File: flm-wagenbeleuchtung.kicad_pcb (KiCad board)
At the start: 2 copper layers, 153 x 9.4 mm, 31 parts

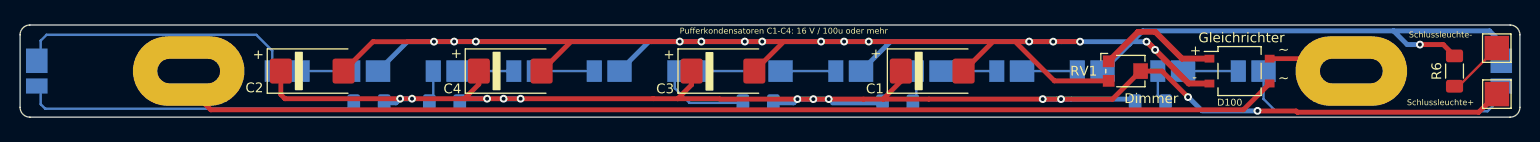
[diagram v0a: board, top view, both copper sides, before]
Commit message: v2
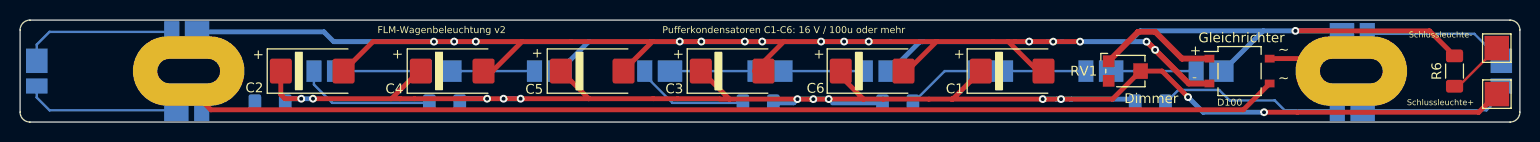
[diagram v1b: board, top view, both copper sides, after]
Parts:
- added C5: 200u, Capacitor_Tantalum_SMD:CP_EIA-7343-31_Kemet-D_Pad2.25x2.55mm_HandSolder, F.Cu at (128.4, 124.7)
- added C6: 200u, Capacitor_Tantalum_SMD:CP_EIA-7343-31_Kemet-D_Pad2.25x2.55mm_HandSolder, F.Cu at (156.9, 124.7)
- moved D32 25.5 mm to (71.7, 124.7), turned to -90 degrees
- moved D42 25.3 mm to (221.1, 124.7), turned to -90 degrees
- moved D31 18.9 mm to (87.0, 120.7)
- moved D43 18.7 mm to (205.9, 128.7)
- moved D33 15.8 mm to (87.0, 128.7), turned to 0 degrees
- moved D41 15.7 mm to (205.9, 120.9), turned to 0 degrees
- moved D23 12.2 mm to (101.5, 124.7)
- moved D1 12.1 mm to (191.5, 124.7)
- moved R4 10.1 mm to (95.5, 127.9)
- moved D22 9.14 mm to (112.8, 124.7)
- moved D2 9.09 mm to (180.2, 124.7)
- moved C1 8.15 mm to (171.2, 124.7)
- moved D21 6.10 mm to (124.0, 124.7)
- moved D3 6.05 mm to (169.0, 124.7)
- moved C4 5.92 mm to (114.1, 124.7)
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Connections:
- RV1 pad 3: GND -> unconnected-(RV1-Pad3)
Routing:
- net Net-(D33-Pad2): track 34.2 -> 5.74 mm
- net Net-(D43-Pad2): track 3.57 -> 18.9 mm
- net Net-(D41-Pad2): track 29.2 -> 14.8 mm
- net Net-(D32-Pad2): track 28.7 -> 16.0 mm
- net Net-(D23-Pad2): track 3.41 -> 13.9 mm
- net Net-(D31-Pad2): track 5.64 -> 16.0 mm
- net Net-(D42-Pad2): track 5.64 -> 15.7 mm
- net GND: track 250.5 -> 260.3 mm
- net VCC: track 169.5 -> 178.2 mm
- net Net-(D3-Pad2): track 3.39 -> 7.74 mm
- net Net-(D21-Pad2): track 5.64 -> 8.67 mm
- net Net-(D22-Pad2): track 5.64 -> 8.67 mm
- net Net-(D2-Pad2): track 5.64 -> 8.67 mm
- net Net-(D12-Pad2): track 5.64 -> 8.67 mm
- net Net-(D1-Pad2): track 5.64 -> 8.67 mm
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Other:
- board size 153 x 9.4 mm -> 153 x 10.4 mm
- board text added: "FLM-Wagenbeleuchtung v2"
- board text added: "Pufferkondensatoren C1-C6: 16 V / 100u oder mehr"
- board text removed: "Pufferkondensatoren C1-C4: 16 V / 100u oder mehr"
